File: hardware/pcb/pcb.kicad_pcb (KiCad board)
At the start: 2 copper layers, 26.7 x 56.6 mm, 28 parts, among them J1 L_GPIO, J2 R_GPIO, U1 ESP32-C3-WROOM-02, U3 TPS62291

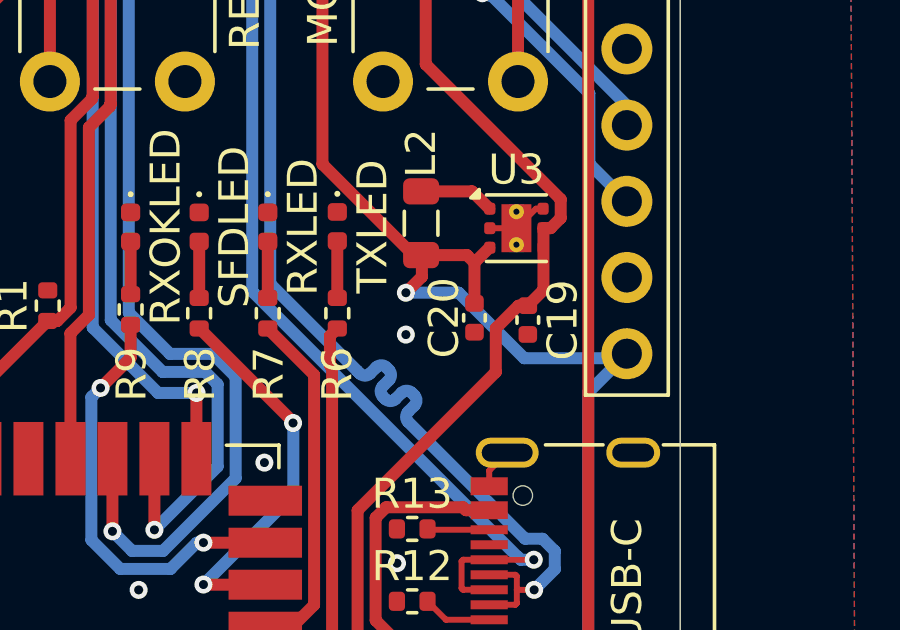
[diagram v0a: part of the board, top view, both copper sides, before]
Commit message: PCB progress
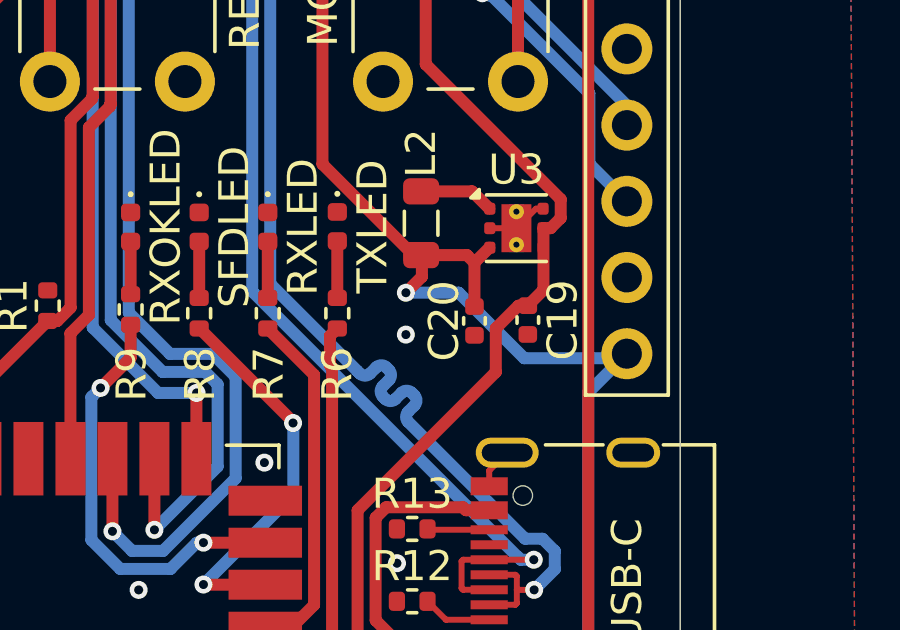
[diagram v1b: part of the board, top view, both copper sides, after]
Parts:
- moved C20 0.10 mm to (109.2, 86.1)
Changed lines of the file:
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@@
 	(footprint "Capacitor_SMD:C_0402_1005Metric"
 		(layer "F.Cu")
-		(at 109.22 86.003 -90)
+		(at 109.22 86.106 -90)
 		(descr "Capacitor SMD 0402 (1005 Metric), square (rectangular) end terminal, IPC-7351 nominal, (Body size source: IPC-SM-782 page 76, https://www.pcb-3d.com/wordpress/wp-content/uploads/ipc-sm-782a_amendment_1_and_2.pdf), generated with kicad-footprint-generator")
 		(tags "capacitor")
@@
 	)
 	(segment
-		(start 109.22 85.523)
-		(end 109.22 84.1635)
-		(width 0.4)
-		(layer "F.Cu")
-		(net 4)
-	)
-	(segment
 		(start 107.4674 84.6346)
 		(end 107.4674 83.9135)
@@
 		(width 0.4)
 		(layer "F.Cu")
+		(net 4)
+	)
+	(segment
+		(start 109.22 85.626)
+		(end 109.22 84.1635)
+		(width 0.4)
+		(layer "F.Cu")
